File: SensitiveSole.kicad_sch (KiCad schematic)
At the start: 13 parts, among them U1 CD74HC4067SM, U2 CD74HC4067SM

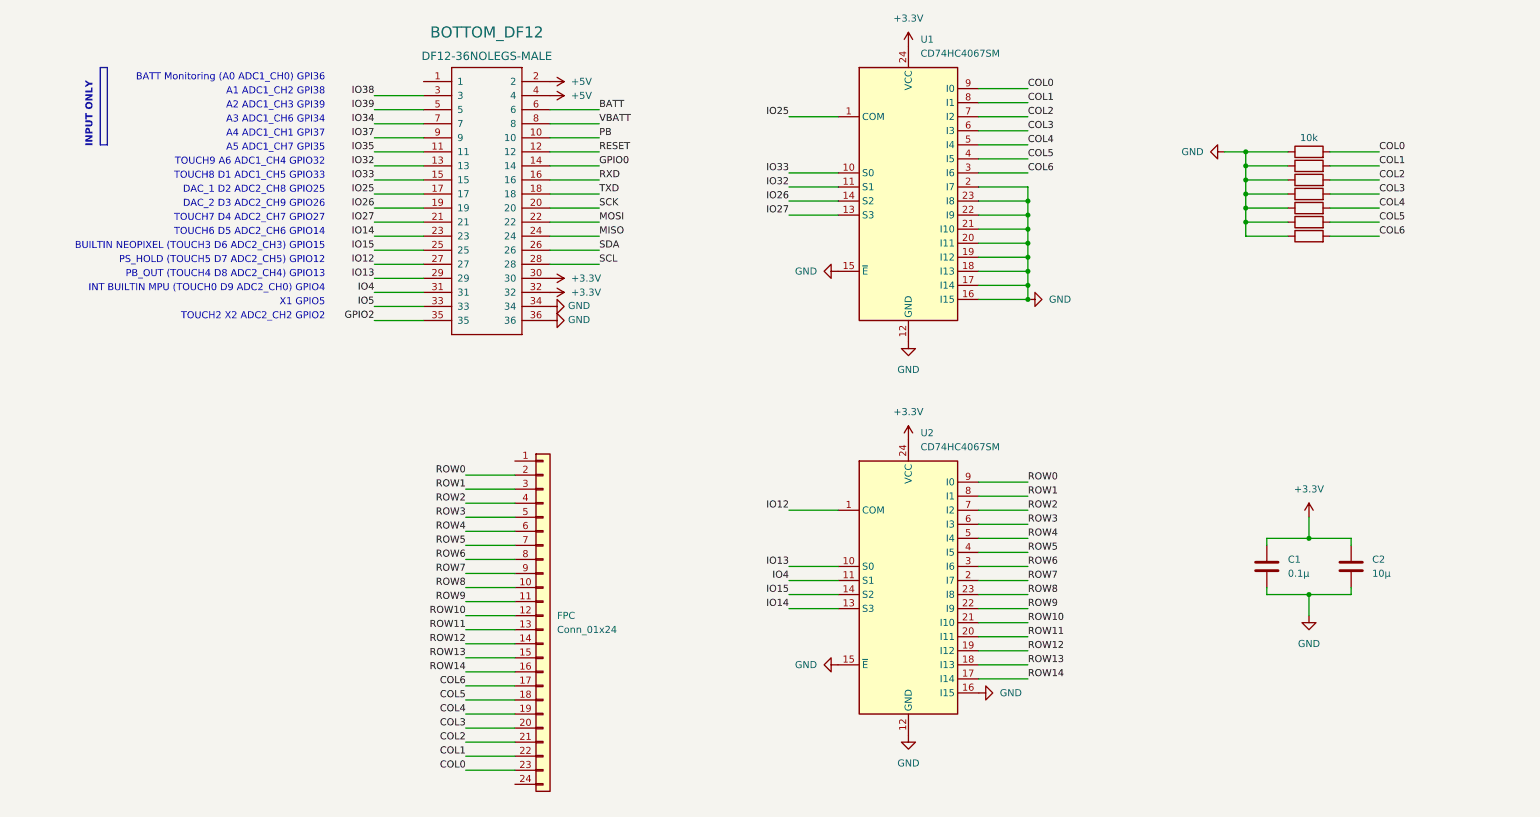
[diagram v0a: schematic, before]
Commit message: base clean
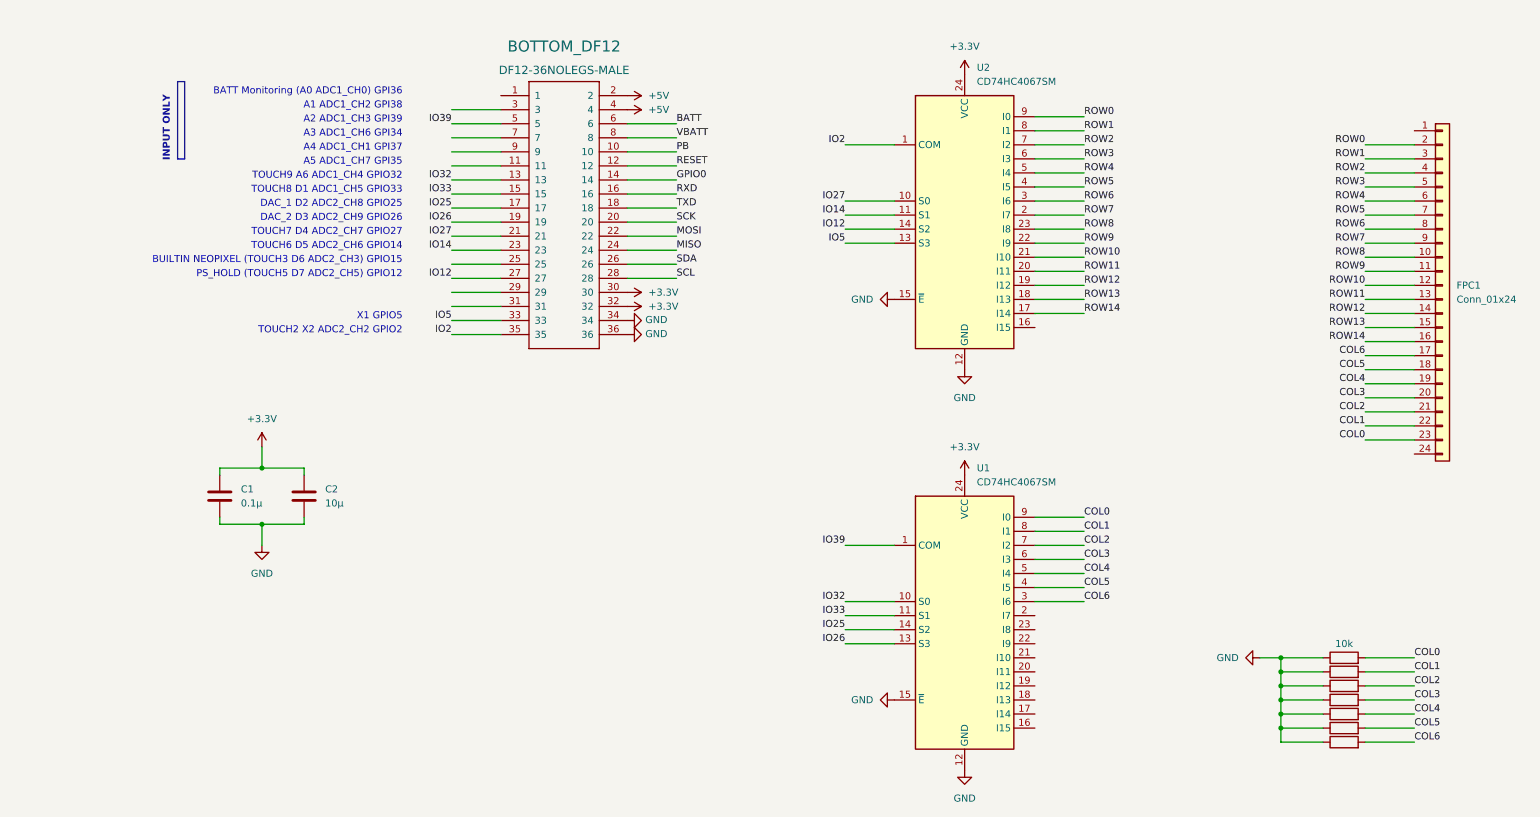
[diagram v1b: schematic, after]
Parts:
- renumbered FPC to FPC1
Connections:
- net GND: no longer U1.16 (I15), U1.17 (I14), U1.18 (I13), U1.19 (I12), U1.2 (I7), U1.20 (I11), U1.21 (I10), U1.22 (I9), U1.23 (I8), U2.16 (I15)
- net IO12: now also U2.14 (S2); no longer U2.1 (COM)
- net IO14: now also U2.11 (S1); no longer U2.13 (S3)
- net IO25: now also U1.14 (S2); no longer U1.1 (COM)
- net IO26: now also U1.13 (S3); no longer U1.14 (S2)
- net IO27: now also U2.10 (S0); no longer U1.13 (S3)
- net IO32: now also U1.10 (S0); no longer U1.11 (S1)
- net IO33: now also U1.11 (S1); no longer U1.10 (S0)
- net IO39: now also U1.1 (COM)
- net IO5: now also U2.13 (S3)
- net GPIO2 renamed IO2
- net IO2: now also U2.1 (COM)
- net IO13: no longer names the net of BOTTOM_DF12.29
- net IO13: no longer U2.10 (S0)
- net IO15: no longer names the net of BOTTOM_DF12.25
- net IO15: no longer U2.14 (S2)
- net IO34: no longer names the net of BOTTOM_DF12.7
- net IO35: no longer names the net of BOTTOM_DF12.11
- net IO37: no longer names the net of BOTTOM_DF12.9
- net IO38: no longer names the net of BOTTOM_DF12.3
- net IO4: no longer names the net of BOTTOM_DF12.31
- net IO4: no longer U2.11 (S1)
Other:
- note removed: "INT BUILTIN MPU (TOUCH0 D9 ADC2_CH0) GPIO4"
- note removed: "PB_OUT (TOUCH4 D8 ADC2_CH4) GPIO13"
- moved on the sheet: BOTTOM_DF12, C1, C2, FPC1, U1, U2
